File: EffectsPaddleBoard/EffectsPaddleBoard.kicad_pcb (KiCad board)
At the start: 4 copper layers, 89.6 x 66.6 mm, 94 parts, among them J1 Conn_01x03_Pin, J2 Conn_01x06_Pin, J3 Barrel_Jack, J4 Conn_01x04_Pin, J5 AudioJack2, J6 AudioJack2, SW1 SW_SPDT, SW2 SW_Push, SW4 SW_Push, U1 STM32F405RGTx, U2 TPS7A0533PDBZ, U3 TLV320AIC3100, U4 TPS54233, U5 TPS7A0533PDBZ, U8 TPS7A0518PDBZ, Y1 16MHz

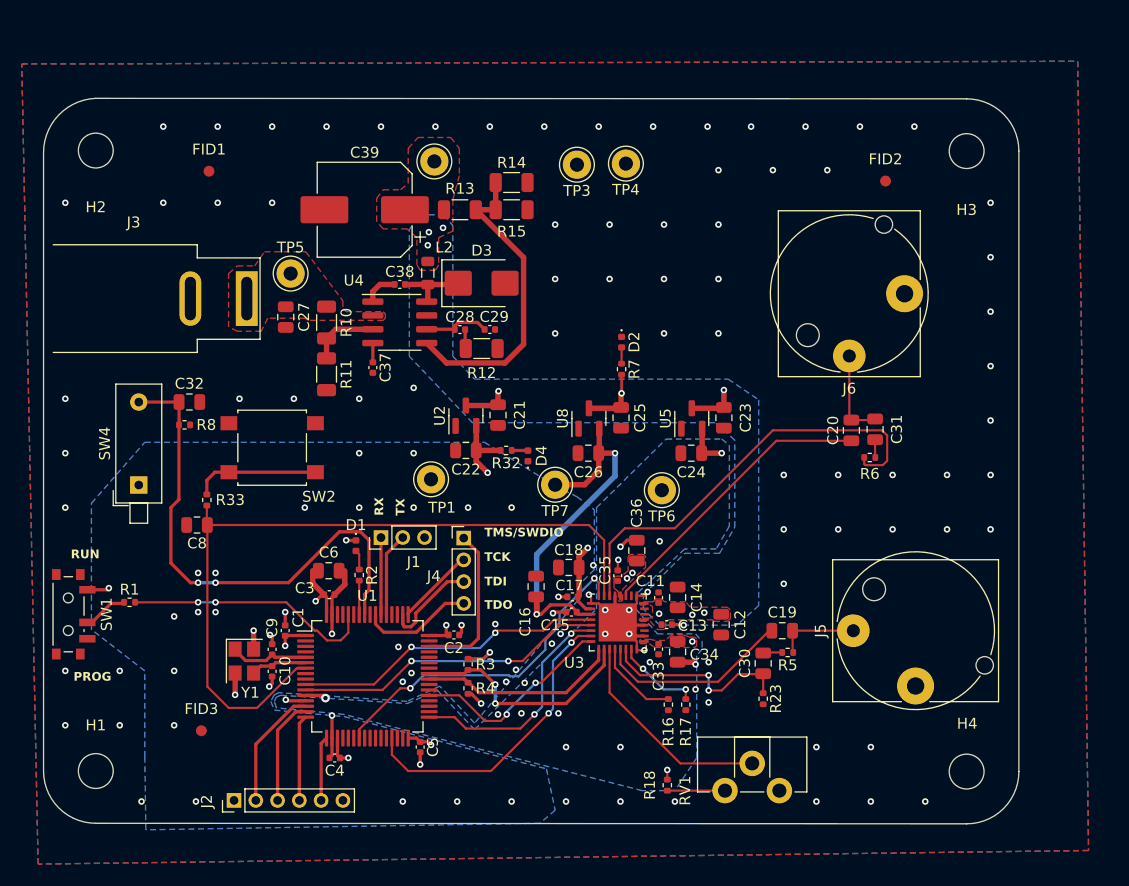
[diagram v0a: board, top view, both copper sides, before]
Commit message: exported symbols and footprints, updated PCB
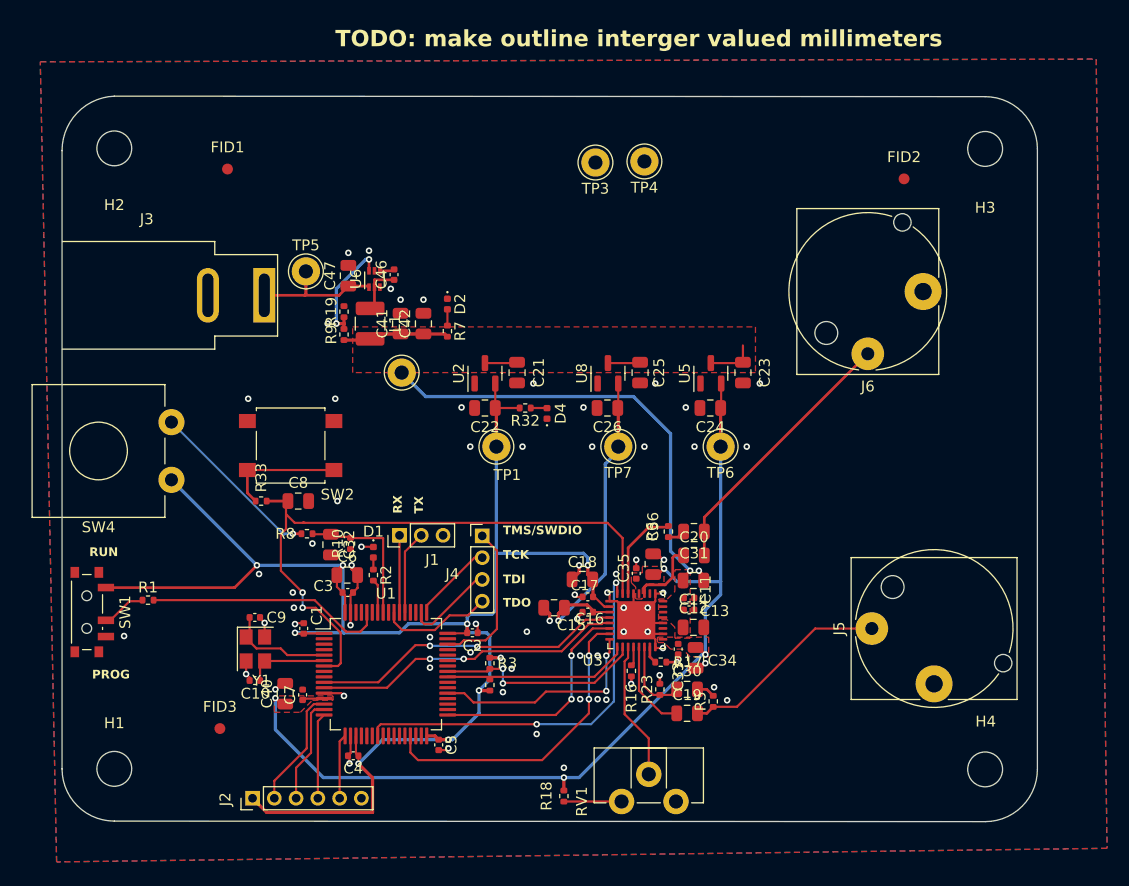
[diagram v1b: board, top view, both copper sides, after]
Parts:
- removed C27: 10u, Capacitor_SMD:C_0805_2012Metric
- removed C28, C29: 220p, Capacitor_SMD:C_0402_1005Metric
- removed C37: 15n, Capacitor_SMD:C_0402_1005Metric
- removed C38: 100n, Capacitor_SMD:C_0402_1005Metric
- removed C39: 470u, Capacitor_SMD:CP_Elec_8x10.5
- removed D3: B230, Diode_SMD:D_SMB
- removed L2: 15u, Inductor_SMD:L_0805_2012Metric
- removed R11: 68.1k, Resistor_SMD:R_1206_3216Metric
- removed R12: 30.9k, Resistor_SMD:R_1206_3216Metric
- removed R13: 10k, Resistor_SMD:R_1206_3216Metric
- removed R14, R15: 3.9k, Resistor_SMD:R_1206_3216Metric
- removed U4: TPS54233, Package_SO:SOIC-8_3.9x4.9mm_P1.27mm
- added C40: 10u, Capacitor_SMD:C_0805_2012Metric, F.Cu at (143.2, 102.1)
- added C41: 22u, Capacitor_SMD:C_0805_2012Metric, F.Cu at (153.8, 68.1)
- added C42: 22u, Capacitor_SMD:C_0805_2012Metric, F.Cu at (155.9, 68.1)
- added C46: 100n, Capacitor_SMD:C_0402_1005Metric, F.Cu at (153.2, 63.6)
- added C47: 10u, Capacitor_SMD:C_0805_2012Metric, F.Cu at (149.0, 63.7)
- added C7: 100n, Capacitor_SMD:C_0402_1005Metric, F.Cu at (144.8, 102.2)
- added L1: 2.2u, Inductor_SMD:L_1210_3225Metric, F.Cu at (151.0, 68.1)
- added R19: 10k, Resistor_SMD:R_0402_1005Metric, F.Cu at (148.6, 67.0)
- added R9: 52.3k, Resistor_SMD:R_0402_1005Metric, F.Cu at (148.6, 69.1)
- added U6: AP62250Z6, Package_TO_SOT_SMD:SOT-563, F.Cu at (151.4, 64.0)
- J3: footprint Connector_BarrelJack:BarrelJack_SwitchcraftConxall_RAPC10U_Horizontal -> Library:BarrelJack_SwitchcraftConxall_RAPC10U_Horizontal
- R10: value 332k -> 220; footprint Resistor_SMD:R_1206_3216Metric -> Resistor_SMD:R_0402_1005Metric
- SW4: footprint Button_Switch_THT:SW_DIP_SPSTx01_Piano_10.8x4.1mm_W7.62mm_P2.54mm -> Button_Switch_THT:SW_CW_GPTS203211B
- moved R10 20.4 mm to (149.2, 88.3), turned to 90 degrees
- moved R6 19.7 mm to (178.4, 87.2), turned to -90 degrees
- moved TP2 19.6 mm to (153.9, 72.6)
- moved C31 19.1 mm to (180.7, 87.2), turned to 0 degrees
- moved C20 18.5 mm to (180.7, 89.4), turned to 0 degrees
- moved C32 18.5 mm to (147.4, 88.4), turned to -90 degrees
- moved D2 16.4 mm to (158.1, 66.3)
- moved R7 16.4 mm to (158.1, 68.8)
- moved R8 15.1 mm to (145.2, 87.4), turned to 180 degrees
- moved C19 11.6 mm to (180.1, 103.9)
- moved C8 9.56 mm to (144.4, 84.4), turned to 0 degrees
- moved R18 9.55 mm to (168.8, 111.5)
- moved RV1 9.55 mm to (174.1, 112.0)
- moved R23 9.53 mm to (177.6, 101.7), turned to 90 degrees
- moved R5 8.18 mm to (182.5, 102.8), turned to 90 degrees
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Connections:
- R10 pad 1: /Barreljack_in -> GND
- R10 pad 2: /en5v -> On-Switch
- R8 pad 2: GND -> Net-(R8-Pad2)
- SW4 pad 2: On-Switch -> Net-(R8-Pad2)
- U3 pad 23: unconnected-(U3-SPKM-Pad19) -> unconnected-(U3-SPKM-Pad23)
- U3 pad 26: unconnected-(U3-SPKP-Pad22) -> unconnected-(U3-SPKP-Pad26)
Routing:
- net +3.3V: track 35.8 -> 154.4 mm, vias 10 -> 9
- net +3.3VA: track 6.88 -> 86.5 mm, vias 6 -> 4
- net +5V: track 14.8 -> 65.0 mm, vias 9 -> 1
- net On-Switch: track 47.0 -> 13.0 mm, vias 2 -> 0
- net Net-(U3-HPR): track 40.0 -> 8.58 mm
- net /fb5v: track 28.9 -> 0.00 mm
- net /Codec/HPL: track 26.9 -> 6.46 mm
- net /Codec/AudioOutBoard: track 8.19 -> 24.8 mm
- net Net-(R8-Pad2): track 0.00 -> 16.5 mm, vias 0 -> 1
- net /Barreljack_in: track 0.00 -> 12.3 mm
- net Net-(C19-Pad2): track 7.60 -> 19.2 mm
- net Codec_Reset: track 70.1 -> 58.8 mm, vias 0 -> 2
- net /Codec/Analog_In_R: track 18.1 -> 7.12 mm, vias 2 -> 0
- net /v_fb: track 0.00 -> 10.1 mm, vias 0 -> 2
- net /Codec/Analog_In_L: track 17.9 -> 8.35 mm
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- removed copper zone on B.Cu, net +3.3V
- removed copper zone on B.Cu, net +3.3VA
- removed copper zone on B.Cu, net +5V
- removed copper zone on F.Cu, net /Barreljack_in
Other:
- outline, holes or cut-outs redrawn
- board text added: "TODO: make outline interger valued millimeters"
